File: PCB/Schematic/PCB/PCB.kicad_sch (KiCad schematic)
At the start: 39 parts, among them J1 Conn_01x02_Socket, J2 Conn_01x02_Pin, J3 Conn_01x02_Pin, J4 Conn_01x02_Socket, U1 LM2735X, U1 STM32L476RGTx, U1 TPS63001DRC, U2 FGPMMOPA6H, U8 LM386

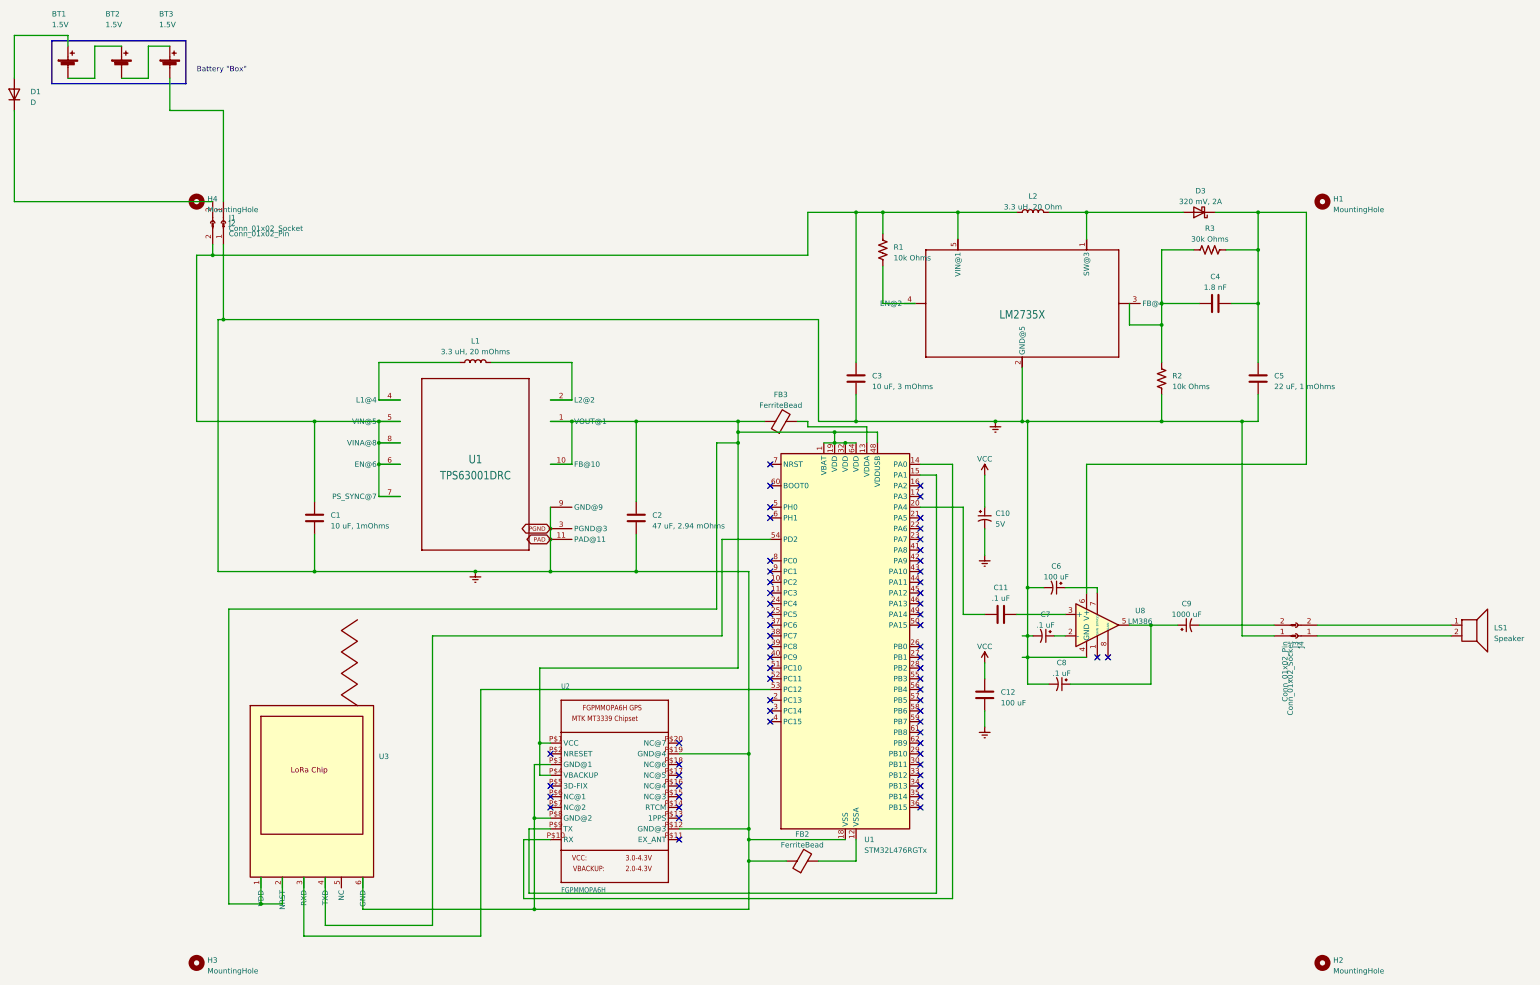
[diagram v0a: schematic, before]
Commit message: Add files via upload
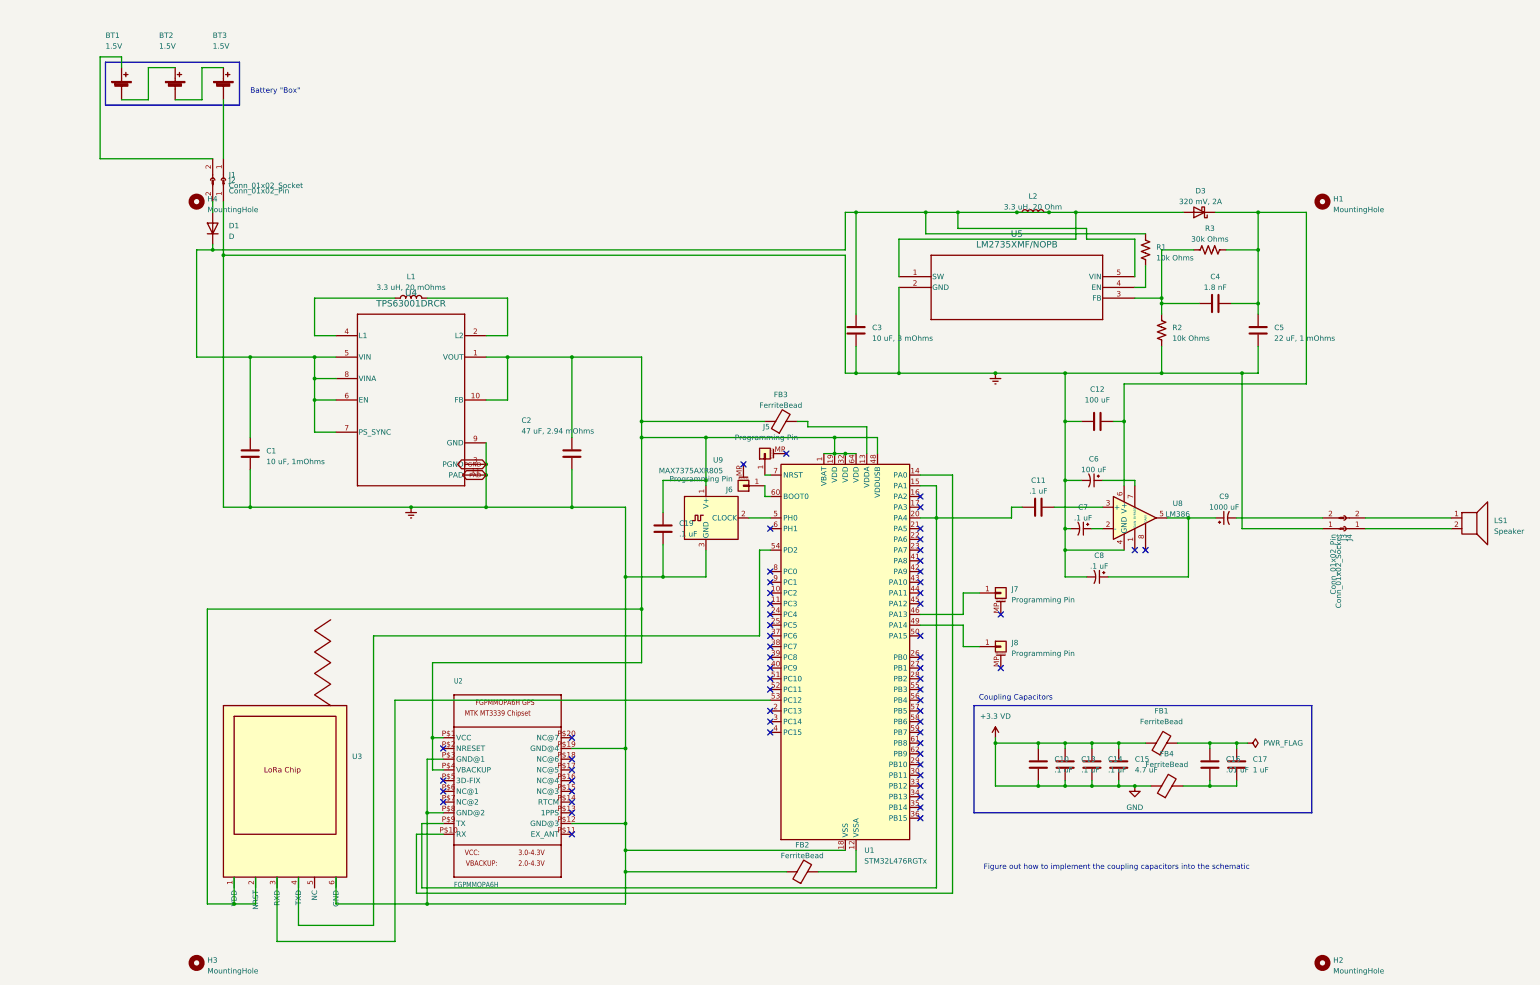
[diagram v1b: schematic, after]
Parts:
- removed C10: 5V, symbol Device:C_Polarized_Small_US
- removed U1: TPS63001DRC, Buck-Boost Converter Chip:DRC0010J, symbol 2024-09-27_13-12-33-eagle-import:TPS63001DRCRTPS63001DRCR
- removed U1: LM2735X, Boost Converter Chip:MF05A, symbol 2024-09-27_13-12-28-eagle-import:LM2735XMF/NOPBLM2735XMF/NOPB
- added C10, C13, C14, C19: .1 uF, symbol Device:C
- added C15: 4.7 uF, symbol Device:C
- added C16: .01 uF, symbol Device:C
- added C17: 1 uF, symbol Device:C
- added FB1, FB4: FerriteBead, symbol Device:FerriteBead
- added J5, J6, J7, J8: Programming Pin, symbol Connector_Generic_MountingPin:Conn_01x01_MountingPin
- added U4: TPS63001DRCR, Buck-Boost:DRC0010J, symbol Buck-Boost Chip:TPS63001DRCR
- added U5: LM2735XMF/NOPB, Boost:MF05A, symbol Boost Chip:LM2735XMF_NOPB
- added U9: MAX7375AXR805, Package_TO_SOT_SMD:SOT-323_SC-70, symbol Oscillator:MAX7375AXR805
- C1, C11, C2, C4: footprint (none) -> Capacitor_SMD:C_0805_2012Metric
- C3, C5, R1, R2, R3: footprint (none) -> Resistor_SMD:R_0805_2012Metric
- C6, C7, C8: footprint (none) -> Polarized Caps (.1 - 100 uF):CAP_UZE_4X3P9_NCH
- C9: footprint (none) -> Polarized Cap 1000 uF:PCAP_10x10-ELECT_NCA
- D1, D3: footprint (none) -> Schottky:Schottky
- FB2, FB3: footprint (none) -> Ferrite_THT:LairdTech_28C0236-0JW-10
- J2, J3: footprint (none) -> Connector_JST:JST_PH_B2B-PH-SM4-TB_1x02-1MP_P2.00mm_Vertical
- L1: footprint (none) -> Inductor_SMD:L_0805_2012Metric
- L2: footprint (none) -> Inductor_SMD:L_TDK_SLF7045
- U8: footprint (none) -> LM386:LM386
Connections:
- net VCC is gone; now on net Earth: C12.2
- net Earth: now also C19.2, U4.11 (PAD), U4.3 (PGND), U4.9 (GND), U5.2 (GND), U9.3 (GND); no longer C12.1
- net at C1.1, C3.1, L2.1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: now also D1.1 (K), D3.2 (A), L2.2, U4.5 (VIN), U4.6 (EN), U4.7 (PS_SYNC), U4.8 (VINA), U5.1 (SW), U5.5 (VIN); no longer J2.2 (Pin_2)
- net at C11.1, U1.20 (PA4): now also U1.15 (PA1), U2.P$9 (TX)
- net at C2.1, FB3.1, U1.1 (VBAT)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: now also C19.1, U4.1 (VOUT), U4.10 (FB), U9.1 (V+)
- net at L1.2: now also U4.2 (L2)
- net at L1.1: now also U4.4 (L1)
- net at D1.2 (A): now also J2.2 (Pin_2); no longer BT1.1 (+)
- net at U1.46 (PA13): now also J7.1 (Pin_1)
- net at U1.49 (PA14): now also J8.1 (Pin_1)
- net at U1.5 (PH0): now also U9.2 (CLOCK)
- net at U1.60 (BOOT0): now also J6.1 (Pin_1)
- net at U1.7 (NRST): now also J5.1 (Pin_1)
- net at C4.1, R2.1, R3.1: now also U5.3 (FB)
- net at C4.2, C5.1, D3.1 (K)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: now also C12.1
- net at R1.2: now also U5.4 (EN)
- net at J1.2 (Pin_2): now also BT1.1 (+); no longer D1.1 (K)
- new net: C16.2, C17.2, FB4.2
- new net: C16.1, C17.1, FB1.2
- new net +3.3 VD: C10.1, C10.2, C13.1, C13.2, C14.1, C14.2, C15.1, C15.2, FB1.1, FB4.1
- no-connect marks 62 -> 61
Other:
- note added: "Coupling Capacitors"
- note added: "Figure out how to implement the coupling capacitors into the schematic"
- moved on the sheet: BT1, BT2, BT3, C1, C11, C12, C2, C3, C5, C6, C7, C8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
